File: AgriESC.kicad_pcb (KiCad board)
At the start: 2 copper layers, 91.9 x 64 mm, 312 parts, among them J1 SUPPLY, J10 GPIO, J11 USB_OTG, J12 HALL_ENC, J2 PH_A, J3 PH_B, J4 PH_C, J6 COMM, J7 SERVO, J8 CAN, J9 SWD, SW1 SW_SPDT, U1 FDMS7698, U10 STM32F405RGT6, U11 DRV8303, U12 TJA1051TK-3, U13 LMR16006YQ, U14 MCP1700-3302E_SOT23, U15 MCP1700-3302E_SOT23, U2 FDMS7698, U3 FDMS7698, U4 FDMS7698, U5 FDMS7698, U6 FDMS7698, U7 MAX9920, U8 MAX9920, U9 MAX9920, Y1 8M Resonator

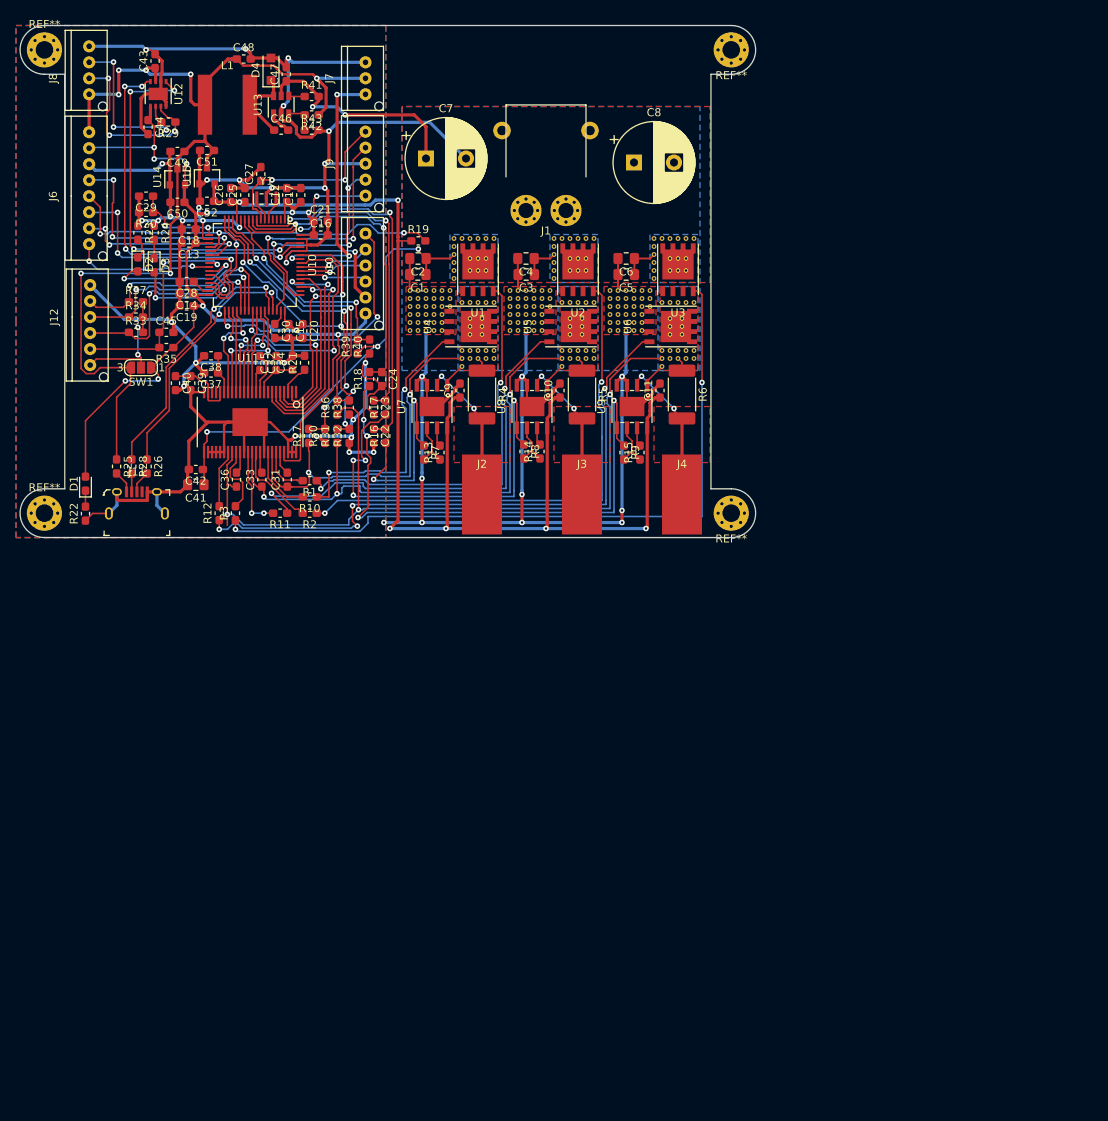
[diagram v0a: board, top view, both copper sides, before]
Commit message: Cleaning routing
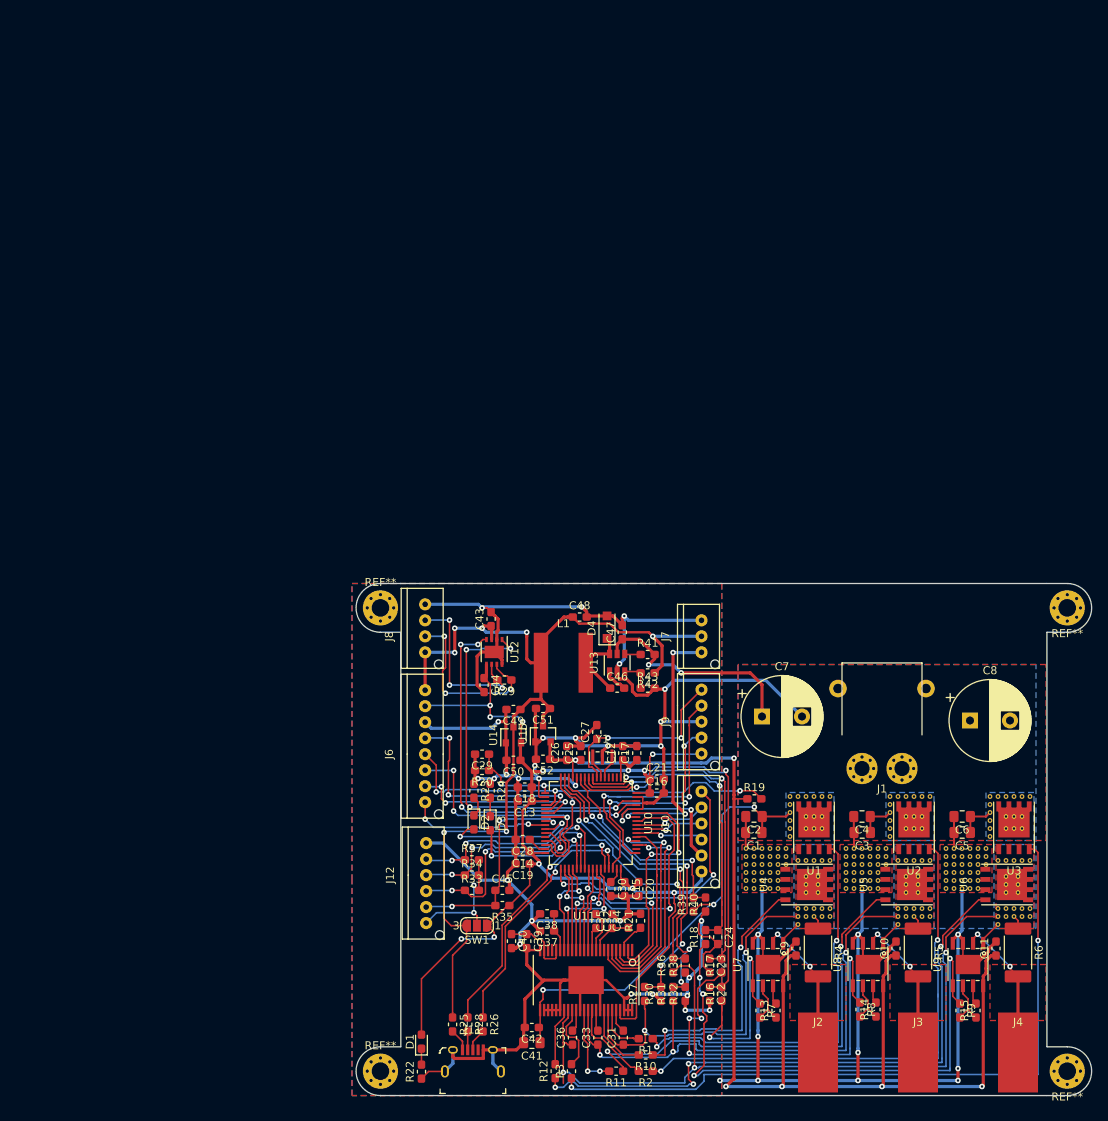
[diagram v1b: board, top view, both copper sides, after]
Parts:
- removed the REF** at (152.9, -5.08)
- removed the REF** at (152.9, 52.8)
- removed the REF** at (67.1, 52.8)
- added REF**: MountingHole_2.2mm_M2_Pad_Via, Mounting_Holes:MountingHole_2.2mm_M2_Pad_Via, F.Cu at (194.9, 64.7)
- added REF**: MountingHole_2.2mm_M2_Pad_Via, Mounting_Holes:MountingHole_2.2mm_M2_Pad_Via, F.Cu at (194.9, 122.6)
- added REF**: MountingHole_2.2mm_M2_Pad_Via, Mounting_Holes:MountingHole_2.2mm_M2_Pad_Via, F.Cu at (109.1, 122.6)
- moved C1 81.4 mm to (155.7, 92.8)
- moved C10 81.4 mm to (173.5, 107.2)
- moved C11 81.4 mm to (186.0, 107.2)
- moved C12 81.4 mm to (139.3, 82.8)
- moved C13 81.4 mm to (127.1, 88.8)
- moved C14 81.4 mm to (126.8, 95.2)
- moved C15 81.4 mm to (139.6, 99.8)
- moved C16 81.4 mm to (143.6, 87.8)
- moved C17 81.4 mm to (141.1, 82.8)
- moved C18 81.4 mm to (127.1, 87.1)
- moved C19 81.4 mm to (126.8, 96.7)
- moved C2 81.4 mm to (155.8, 90.8)
- moved C20 81.4 mm to (141.3, 99.8)
- moved C21 81.4 mm to (143.6, 86.1)
- moved C22 81.4 mm to (150.2, 112.9)
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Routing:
- net +5V: track 129.3 -> 121.3 mm
- net HALL_3: track 28.5 -> 28.0 mm, vias 2 -> 3
- net HALL_2: track 27.5 -> 27.6 mm, vias 2 -> 3
- net HALL_1: vias 2 -> 3
- net TEMP_MOTOR: vias 2 -> 3
